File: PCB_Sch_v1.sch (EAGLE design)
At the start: 12 parts, among them U1 ESP32-WROOM-32D, U2 UG-2828GDEDF11

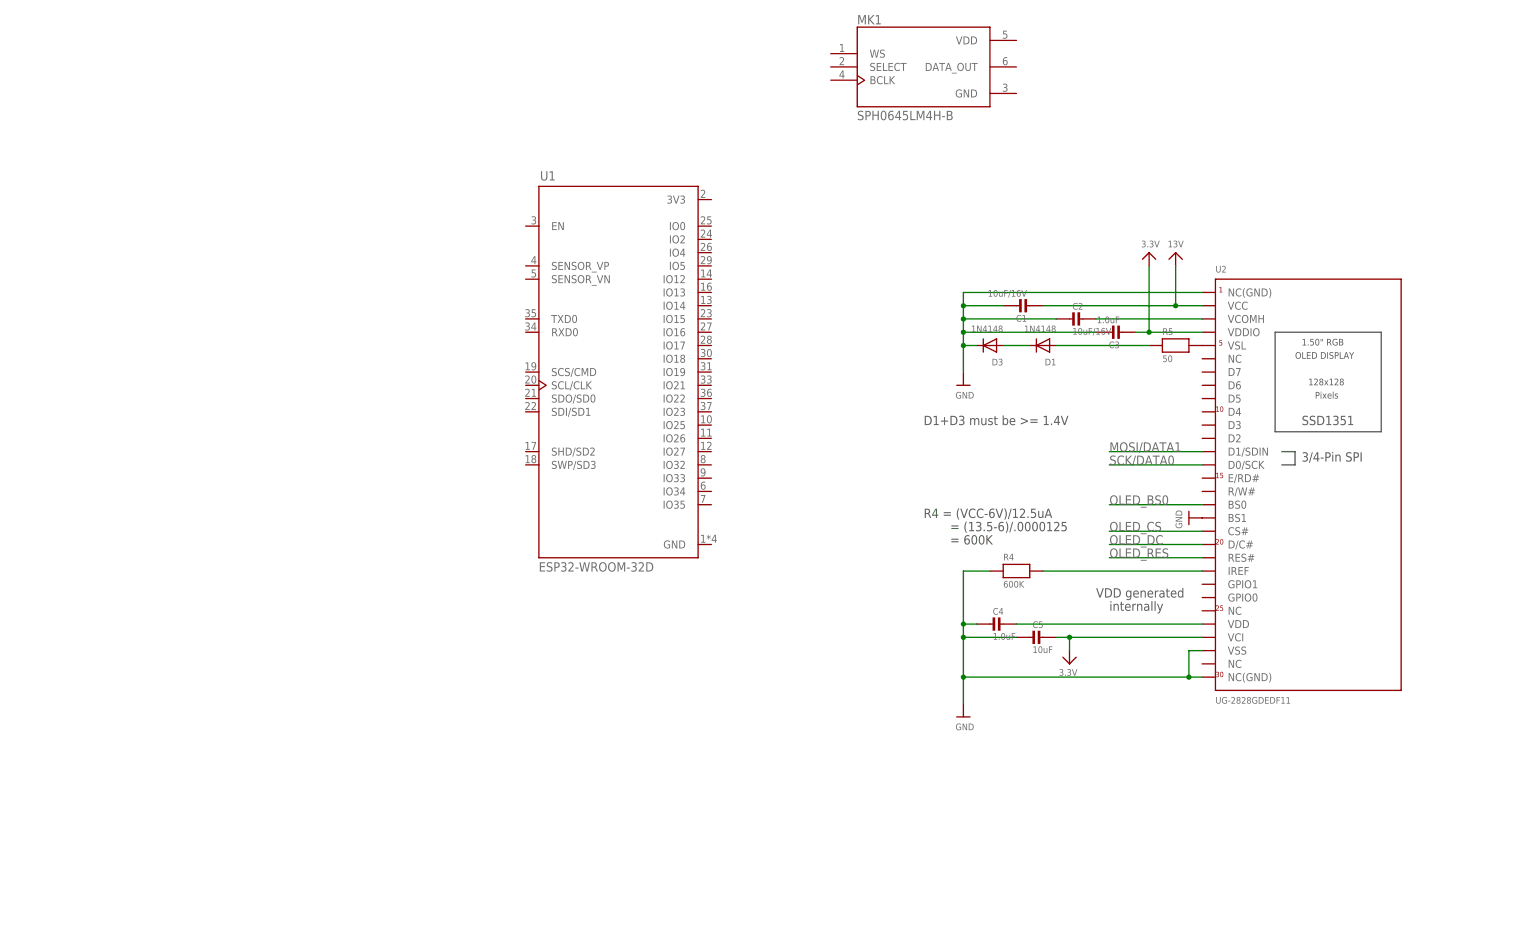
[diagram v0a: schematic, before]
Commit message: Progress made on 03/18/2019
Connectted excitor and microphone, also contruct some wires for buttons
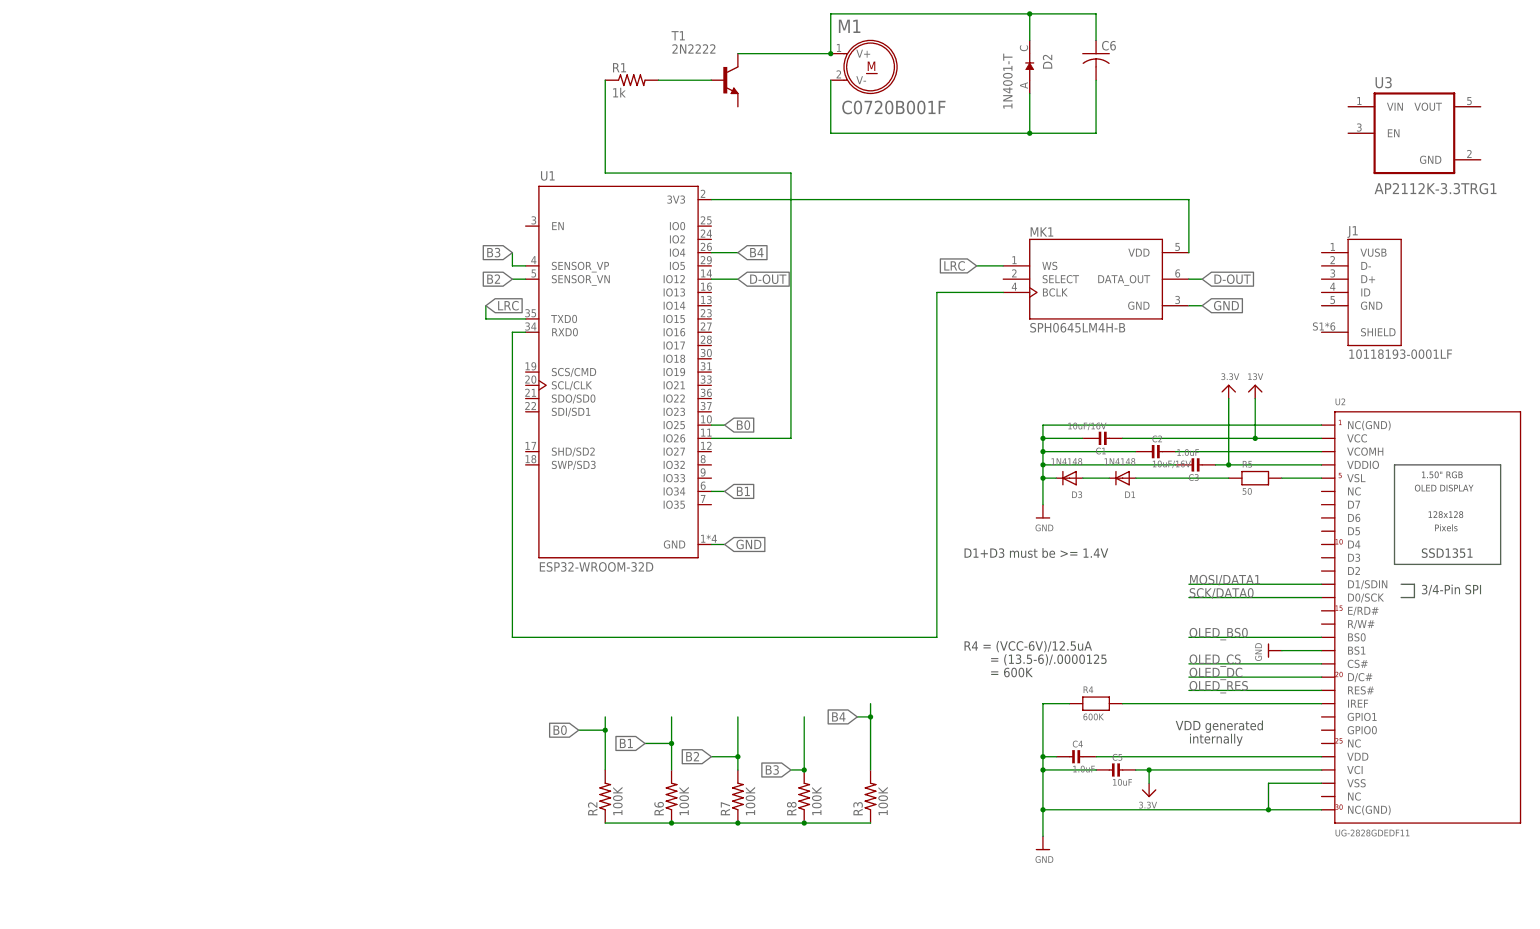
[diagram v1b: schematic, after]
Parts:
- added C6: (no value), adafruit:C-USC0805
- added D2: 1N4001-T, 1N4001-T:1N4001-T
- added J1: 10118193-0001LF, 10118193-0001LF:10118193-0001LF
- added M1: C0720B001F, C0720B001F:C0720B001F
- added R1: 1k, adafruit:R-US_R0805
- added R2, R3, R6, R7, R8: 100K, adafruit:R-US_R0805
- added T1: 2N2222, adafruit:2N2222
- added U3: AP2112K-3.3TRG1, AP2112K-3.3TRG1:AP2112K-3.3TRG1
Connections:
- new net B0: R2.2, U1.IO25
- new net B1: R6.2, U1.IO34
- new net B2: R7.2, U1.SENSOR_VN
- new net B3: R8.2, U1.SENSOR_VP
- new net B4: R3.2, U1.IO4
- new net D-OUT: MK1.DATA_OUT, U1.IO12
- new net LRC: MK1.WS, U1.TXD0
- new net N$1: C6.1, D2.C, M1.V+, T1.C
- new net N$10: MK1.BCLK, U1.RXD0
- new net N$2: R1.2, T1.B
- new net N$4: C6.2, D2.A, M1.V-
- new net N$5: MK1.VDD, U1.3V3
- new net N$8: R2.1, R3.1, R6.1, R7.1, R8.1
- new net N$9: R1.1, U1.IO26
- net GND: now also MK1.GND, U1.GND
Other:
- moved on the sheet: C1, C2, C3, C4, C5, D1, D3, MK1, R4, R5, U2

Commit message: Add files via upload
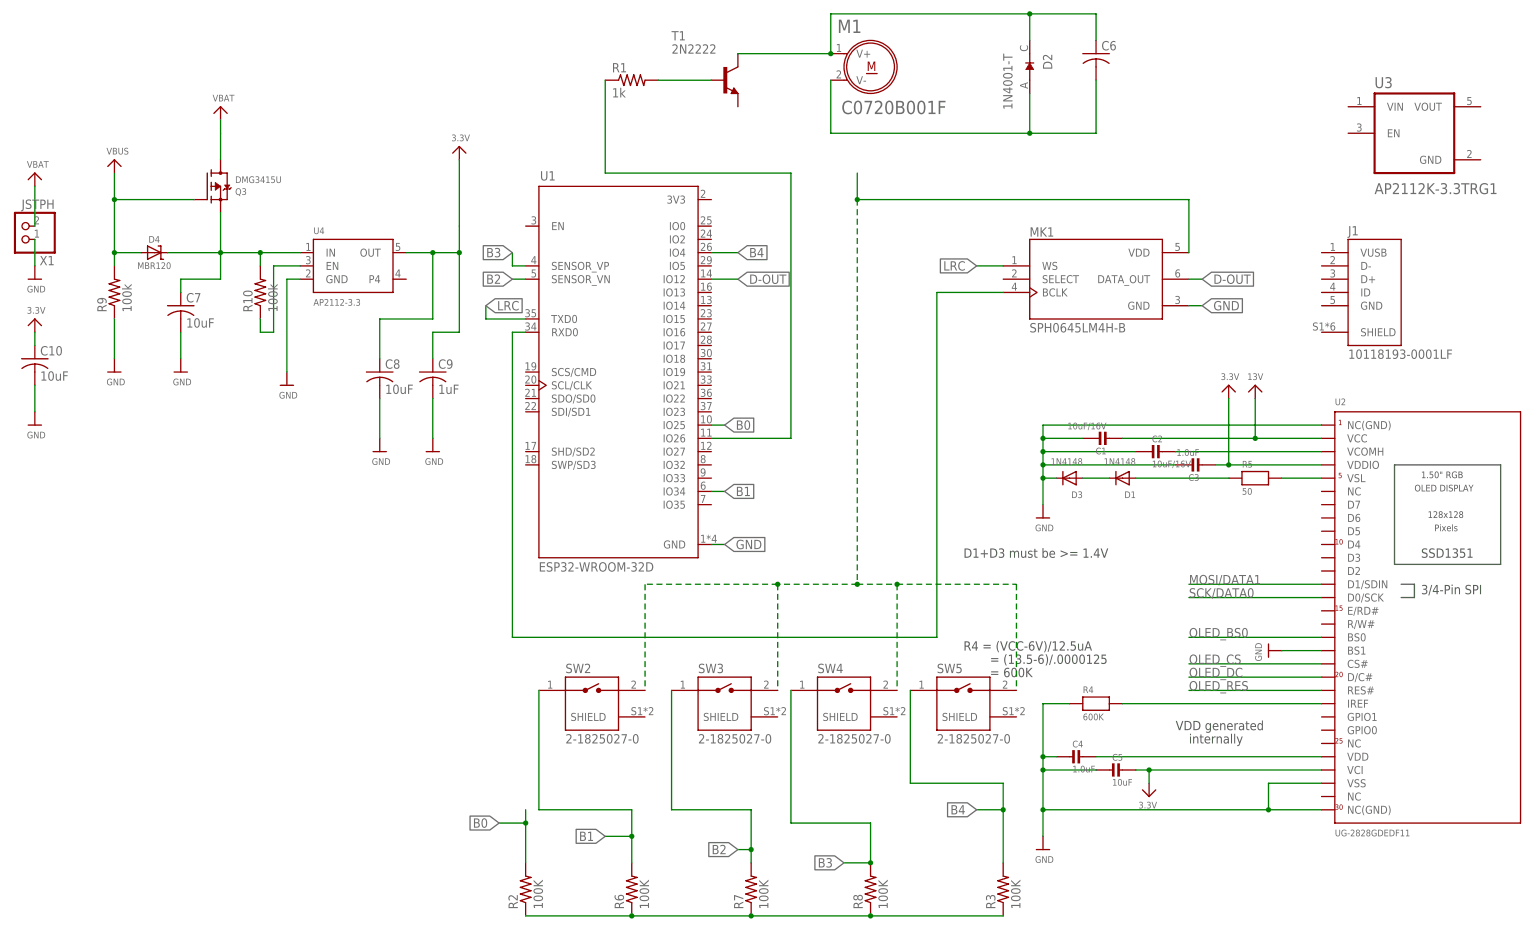
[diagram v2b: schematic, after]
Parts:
- added C10, C7, C8: 10uF, adafruit:C-USC0805
- added C9: 1uF, adafruit:C-USC0805
- added D4: MBR120, microbuilder:DIODE-SCHOTTKYSOD-123
- added Q3: DMG3415U, microbuilder:MOSFET-P
- added R10, R9: 100k, adafruit:R-US_R0805
- added SW2, SW3, SW4, SW5: 2-1825027-0, 2-1825027-0:2-1825027-0
- added U4: AP2112-3.3, microbuilder:VREG_SOT23-5
- added X1: JSTPH, microbuilder:CON_JST_PH_2PIN
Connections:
- new net N$12: C7.1, D4.C, Q3.S, R10.2, U4.IN
- new net N$14: R10.1, U4.EN
- new net N$15: Q3.D
- new net OUT: C8.1, C9.1, U4.OUT
- new net VBAT: X1.2
- new net VBUS: D4.A, Q3.G, R9.2
- net 3.3V: now also C10.1
- net B1: now also SW2.1
- net B2: now also SW3.1
- net B3: now also SW4.1
- net B4: now also SW5.1
- net GND: now also C10.2, C7.2, C8.2, C9.2, R9.1, U4.GND, X1.1
- net N$5: now also SW2.2, SW3.2, SW4.2, SW5.2; no longer U1.3V3
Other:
- moved on the sheet: R2, R3, R6, R7, R8
